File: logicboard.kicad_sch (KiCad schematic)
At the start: 23 parts, among them SW1 BOOT, SW2 RST, U1 STM32F405RGT7, Y1 Crystal

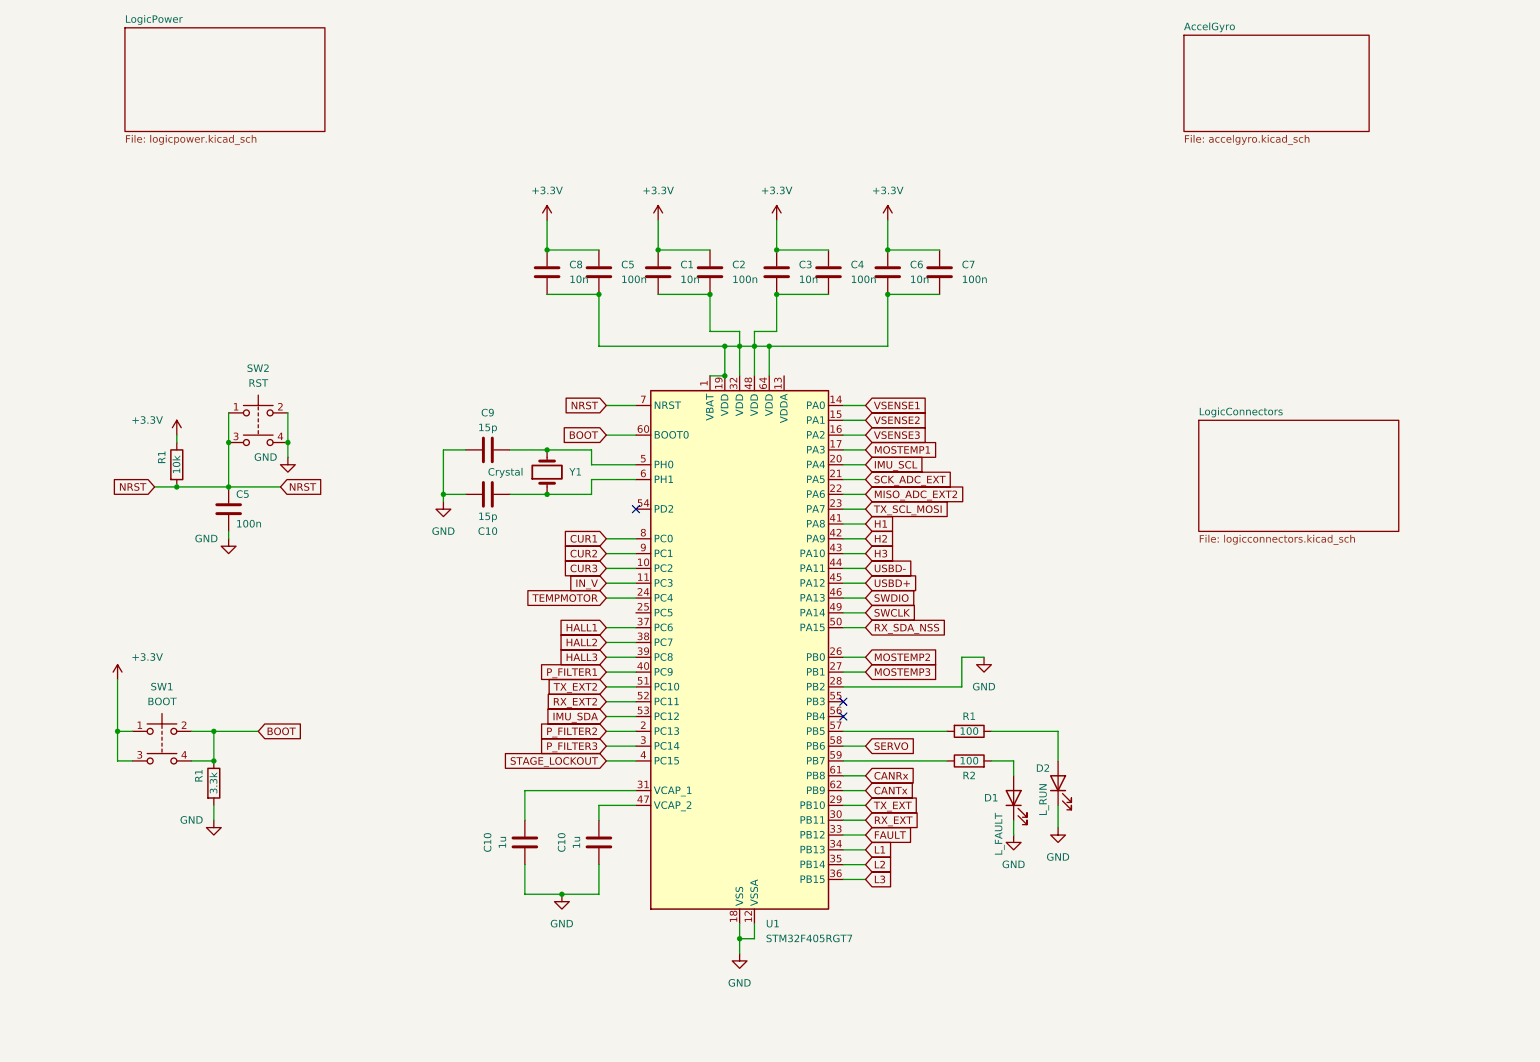
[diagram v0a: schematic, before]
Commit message: initial
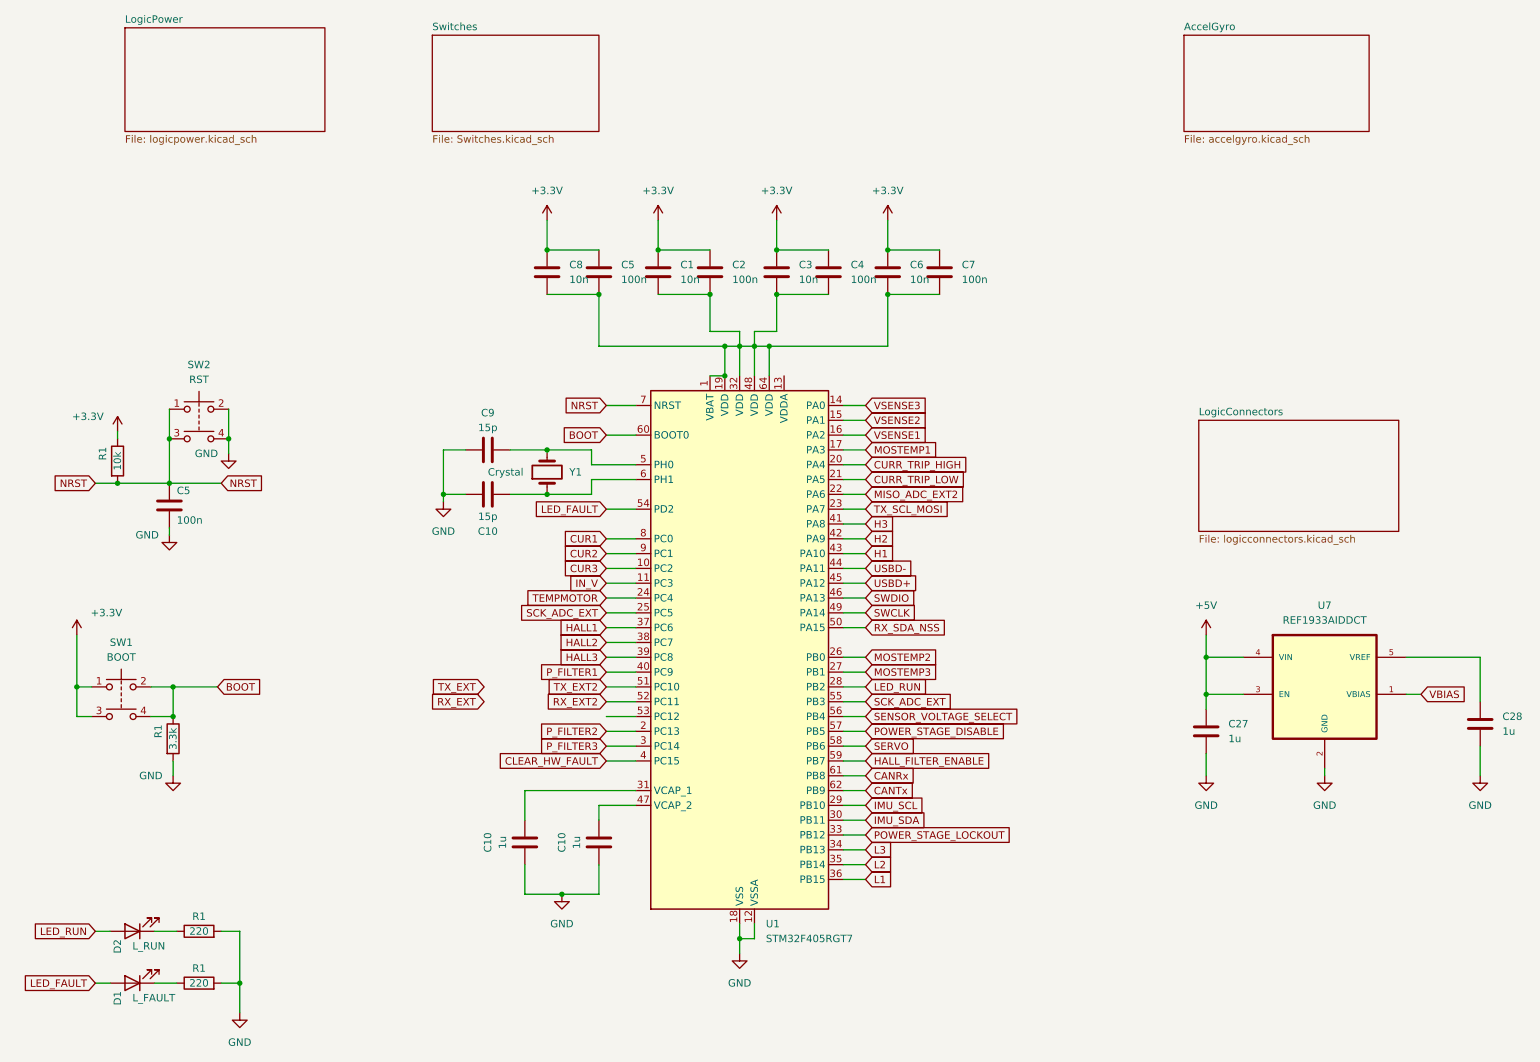
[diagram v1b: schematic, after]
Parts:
- removed R2: 100, symbol Device:R
- added C27, C28: 1u, symbol Device:C
- added R1: 220, symbol Device:R
- added U7: REF1933AIDDCT, SOT95P280X110-5N, symbol GigaVescSymbols:REF1933AIDDCT
- R1: value 100 -> 220
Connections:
- net GND: now also R1.2, C27.2, C28.2, R1.2, U7.2 (GND); no longer D1.1 (K), D2.1 (K), U1.28 (PB2)
- net H1: now also U1.43 (PA10); no longer U1.41 (PA8)
- net H3: now also U1.41 (PA8); no longer U1.43 (PA10)
- net IMU_SCL: now also U1.29 (PB10); no longer U1.20 (PA4)
- net IMU_SDA: now also U1.30 (PB11); no longer U1.53 (PC12)
- net L1: now also U1.36 (PB15); no longer U1.34 (PB13)
- net L3: now also U1.34 (PB13); no longer U1.36 (PB15)
- net RX_EXT: no longer U1.30 (PB11)
- net SCK_ADC_EXT: now also U1.25 (PC5), U1.55 (PB3); no longer U1.21 (PA5)
- net TX_EXT: no longer U1.29 (PB10)
- net VSENSE1: now also U1.16 (PA2); no longer U1.14 (PA0)
- net VSENSE3: now also U1.14 (PA0); no longer U1.16 (PA2)
- net LED_FAULT: now reaches D1.2 (A)
- net LED_FAULT: now also U1.54 (PD2)
- net at R1.1: now also D2.1 (K); no longer D2.2 (A)
- net HALL_FILTER_ENABLE: now reaches U1.59 (PB7)
- net SENSOR_VOLTAGE_SELECT: now reaches U1.56 (PB4)
- net POWER_STAGE_DISABLE: now reaches U1.57 (PB5)
- net POWER_STAGE_DISABLE: no longer R1.2
- net FAULT renamed POWER_STAGE_LOCKOUT
- net STAGE_LOCKOUT renamed CLEAR_HW_FAULT
- new net: D1.1 (K), R1.1
- new net: C28.1, U7.5 (VREF)
- new net +5V: C27.1, U7.3 (EN), U7.4 (VIN)
- new net CURR_TRIP_HIGH: U1.20 (PA4)
- new net CURR_TRIP_LOW: U1.21 (PA5)
- new net LED_RUN: D2.2 (A), U1.28 (PB2)
- new net VBIAS: U7.1 (VBIAS)
- no-connect marks 3 -> 0
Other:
- added sheet Switches (Switches.kicad_sch)
- moved on the sheet: C5, D1, D2, R1, SW1, SW2
